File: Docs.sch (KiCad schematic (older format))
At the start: 0 parts

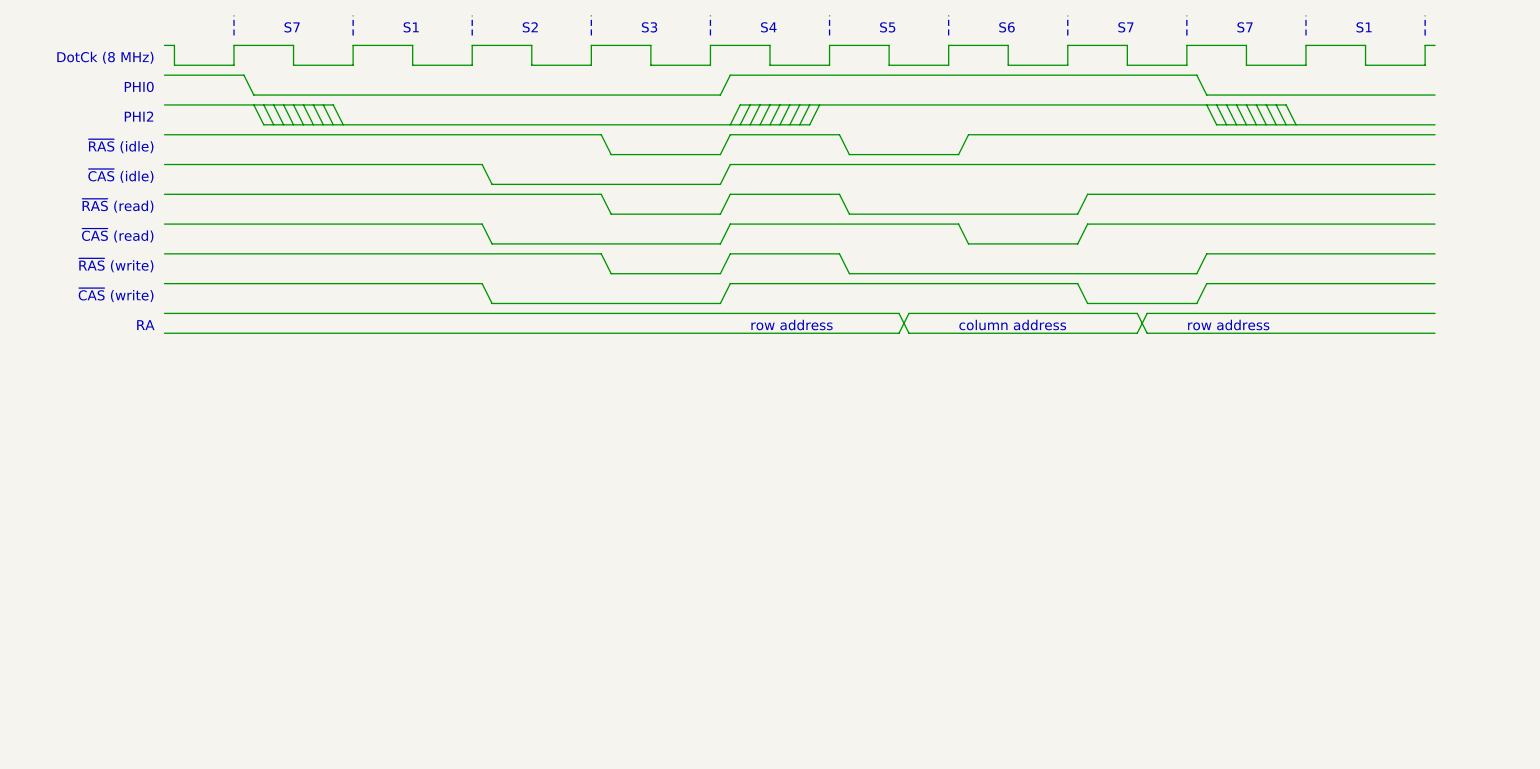
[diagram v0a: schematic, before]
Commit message: idk
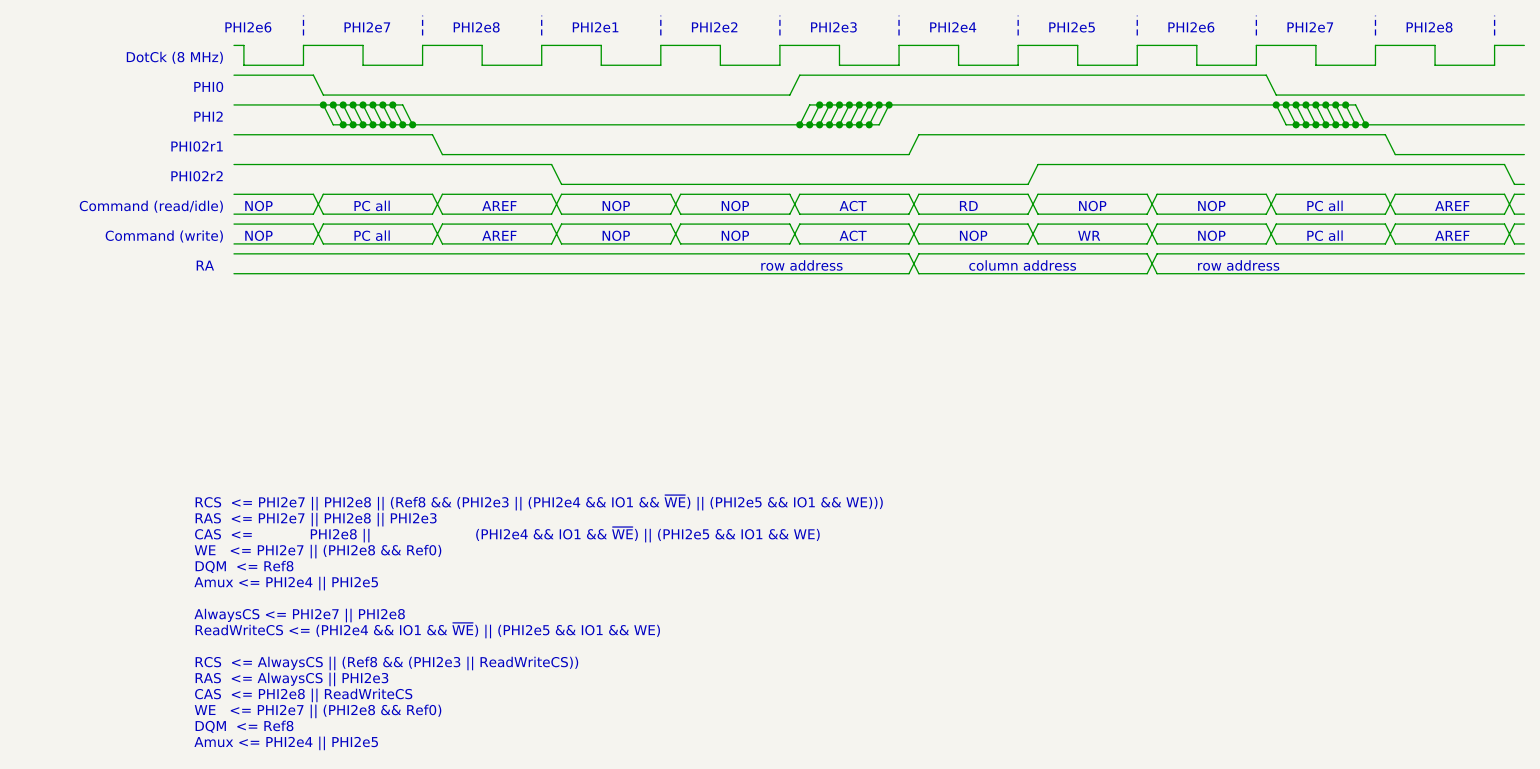
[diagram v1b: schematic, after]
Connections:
- wire segments 143 -> 247
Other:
- note added: "ACT"
- note added: "AREF"
- note added: "Command (read/idle)"
- note added: "Command (write)"
- note added: "NOP"
- note added: "PC all"
- note added: "PHI02r1"
- note added: "PHI02r2"
- note added: "PHI2e1"
- note added: "PHI2e2"
- note added: "PHI2e3"
- note added: "PHI2e4"
- note added: "PHI2e5"
- note added: "PHI2e6"
- note added: "PHI2e7"
- note added: "PHI2e8"
- note added: "RCS <= PHI2e7 || PHI2e8 || (Ref8 && (PHI2e3 || (PHI2e4 && IO1 && ~WE~) || (PHI2e5 && IO1 && WE)))\nRAS <= PHI2e7 || PHI2e8 || PHI2e3\nCAS <= PHI2e8 || (PHI2e4 && IO1 && ~WE~) || (PHI2e5 && IO1 && WE)\nWE <= PHI2e7 || (PHI2e8 && Ref0)\nDQM <= Ref8\nAmux <= PHI2e4 || PHI2e5\n\nAlwaysCS <= PHI2e7 || PHI2e8\nReadWriteCS <= (PHI2e4 && IO1 && ~WE~) || (PHI2e5 && IO1 && WE)\n\nRCS <= AlwaysCS || (Ref8 &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"
- note added: "RD"
- note added: "WR"
- note removed: "S1"
- note removed: "S2"
- note removed: "S3"
- note removed: "S4"
- note removed: "S5"
- note removed: "S6"
- note removed: "S7"
- note removed: "~CAS~ (idle)"
- note removed: "~CAS~ (read)"
- note removed: "~CAS~ (write)"
- note removed: "~RAS~ (idle)"
- note removed: "~RAS~ (read)"
- note removed: "~RAS~ (write)"
